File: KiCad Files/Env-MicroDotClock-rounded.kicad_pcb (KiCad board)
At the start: 2 copper layers, 90 x 65.2 mm, 47 parts, among them IC1 IS31FL3730-QFLS2-TR, IC2 IS31FL3730-QFLS2-TR, IC3 IS31FL3730-QFLS2-TR, IC4 IS31FL3730-QFLS2-TR, M1 Dip-14 Socket, M2 Dip-14 Socket, M3 Dip-14 Socket, M4 Dip-14 Socket, M5 Dip-14 Socket, M6 Dip-14 Socket, M7 Dip-14 Socket, M8 Dip-14 Socket, Q1 2SC1815, SW1 SKRK, SW2 SKRK, SW3 SKRK, SW4 SKRK, U1 Raspberry Pi Pico, U3 DS3231M

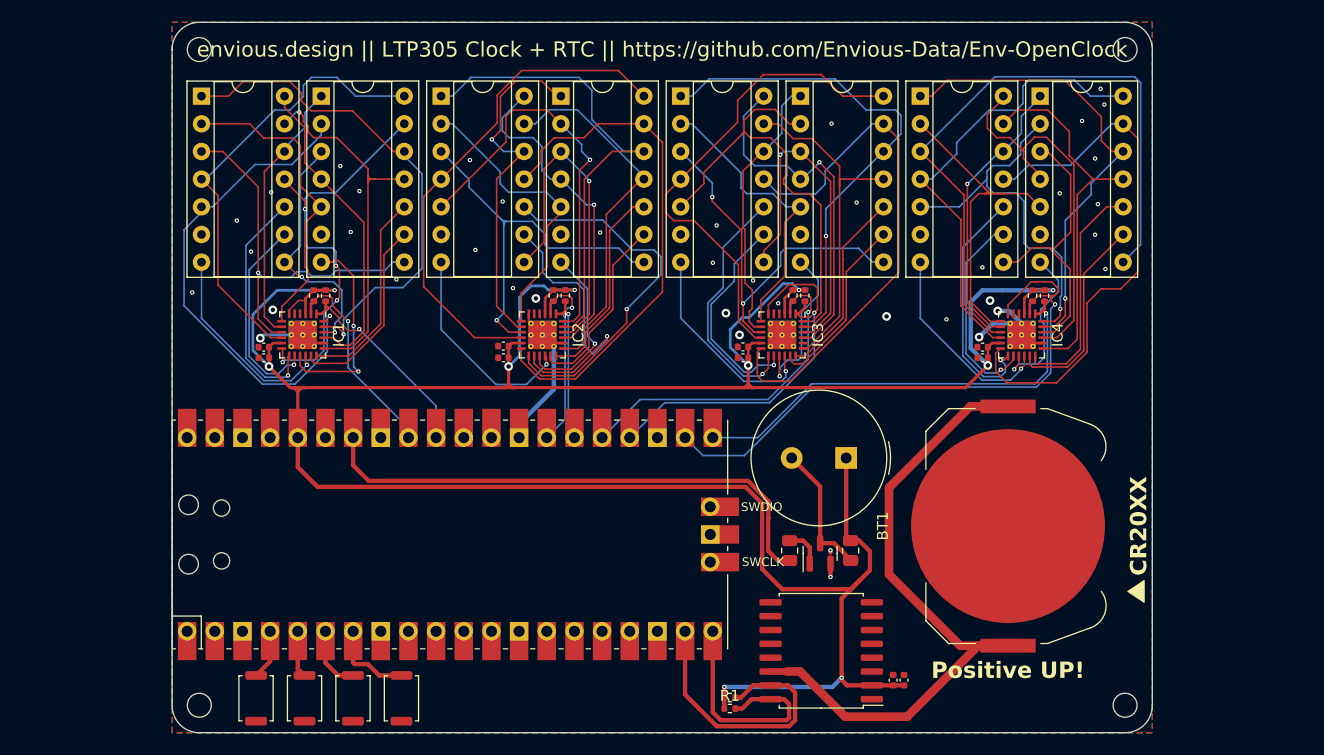
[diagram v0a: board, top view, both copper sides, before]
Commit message: made a roundfied version
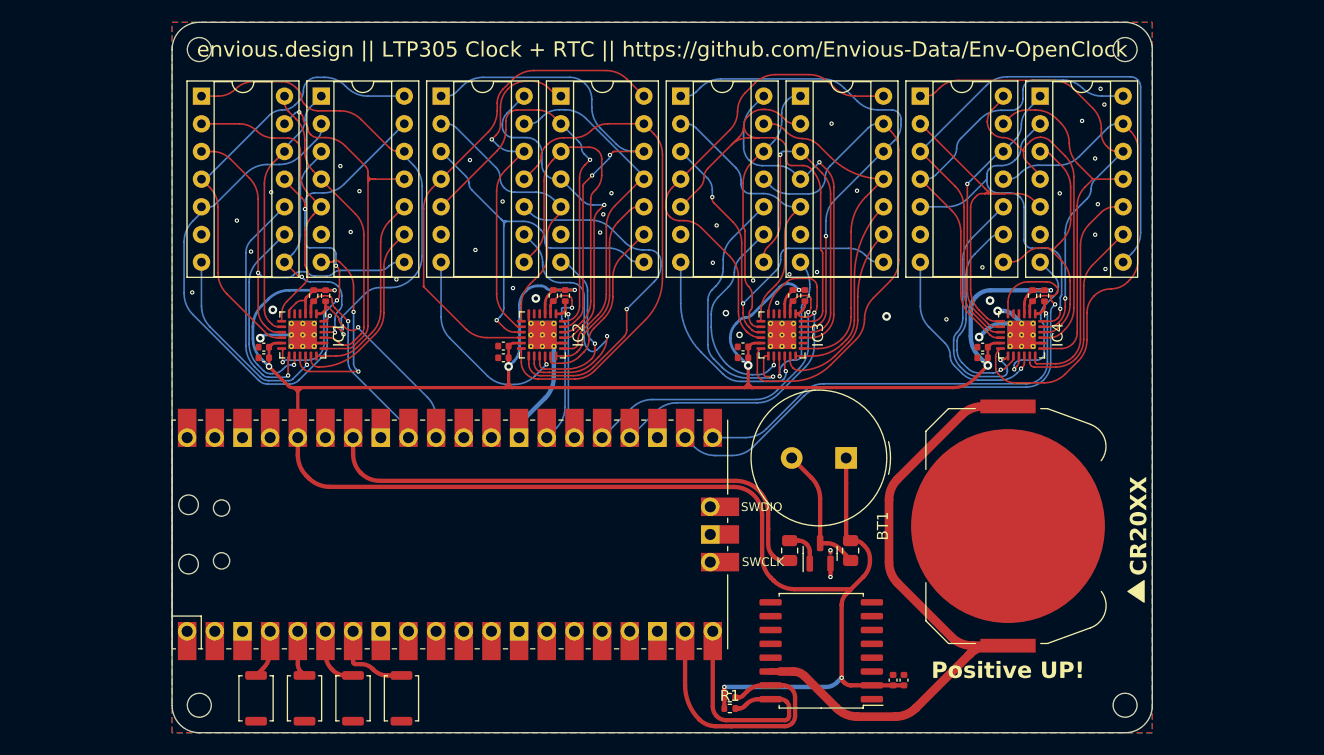
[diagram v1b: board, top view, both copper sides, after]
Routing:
- net +3V3: track 276.8 -> 266.6 mm
- net IC2C3: track 30.6 -> 33.2 mm, vias 1 -> 0
- net IC3R6: track 22.7 -> 25.0 mm
- net IC3C1: track 40.7 -> 42.9 mm
- net IC4R5: track 49.9 -> 48.6 mm
- net IC3C7: track 16.6 -> 17.9 mm
- net IC1R1: track 28.6 -> 27.3 mm
- net IC4R6: track 22.3 -> 23.4 mm
- net IC3R4: track 44.7 -> 43.6 mm
- net IC3R8: track 15.1 -> 14.0 mm
- net IC4R4: track 42.6 -> 41.5 mm
- net IC2C2: track 45.1 -> 44.1 mm, vias 0 -> 2
- net IC4C2: track 43.0 -> 42.0 mm
- net Net-(BT1-+): track 61.8 -> 60.9 mm
- net IC4C1: track 35.1 -> 34.1 mm
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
